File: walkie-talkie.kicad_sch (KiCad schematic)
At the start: 25 parts, among them J1 I2C, U1 ESP32-S3(R8), U10 FS-1540, U11 PJ-327A_5JJ, U12 LIS2DH12TR, U13 MCP73831T-2ACI_OT, U14 ON, U15 AP2112K-3_3TRG1, U16 +, U2 BH-18650-B1BA002, U3 mems-mic, U4 TF-115, U5 SK6812MINI-HS, U6 SK6812MINI-HS, U7 SK6812MINI-HS, U8 SK6812MINI-HS, U9 MAX98357AETE+T

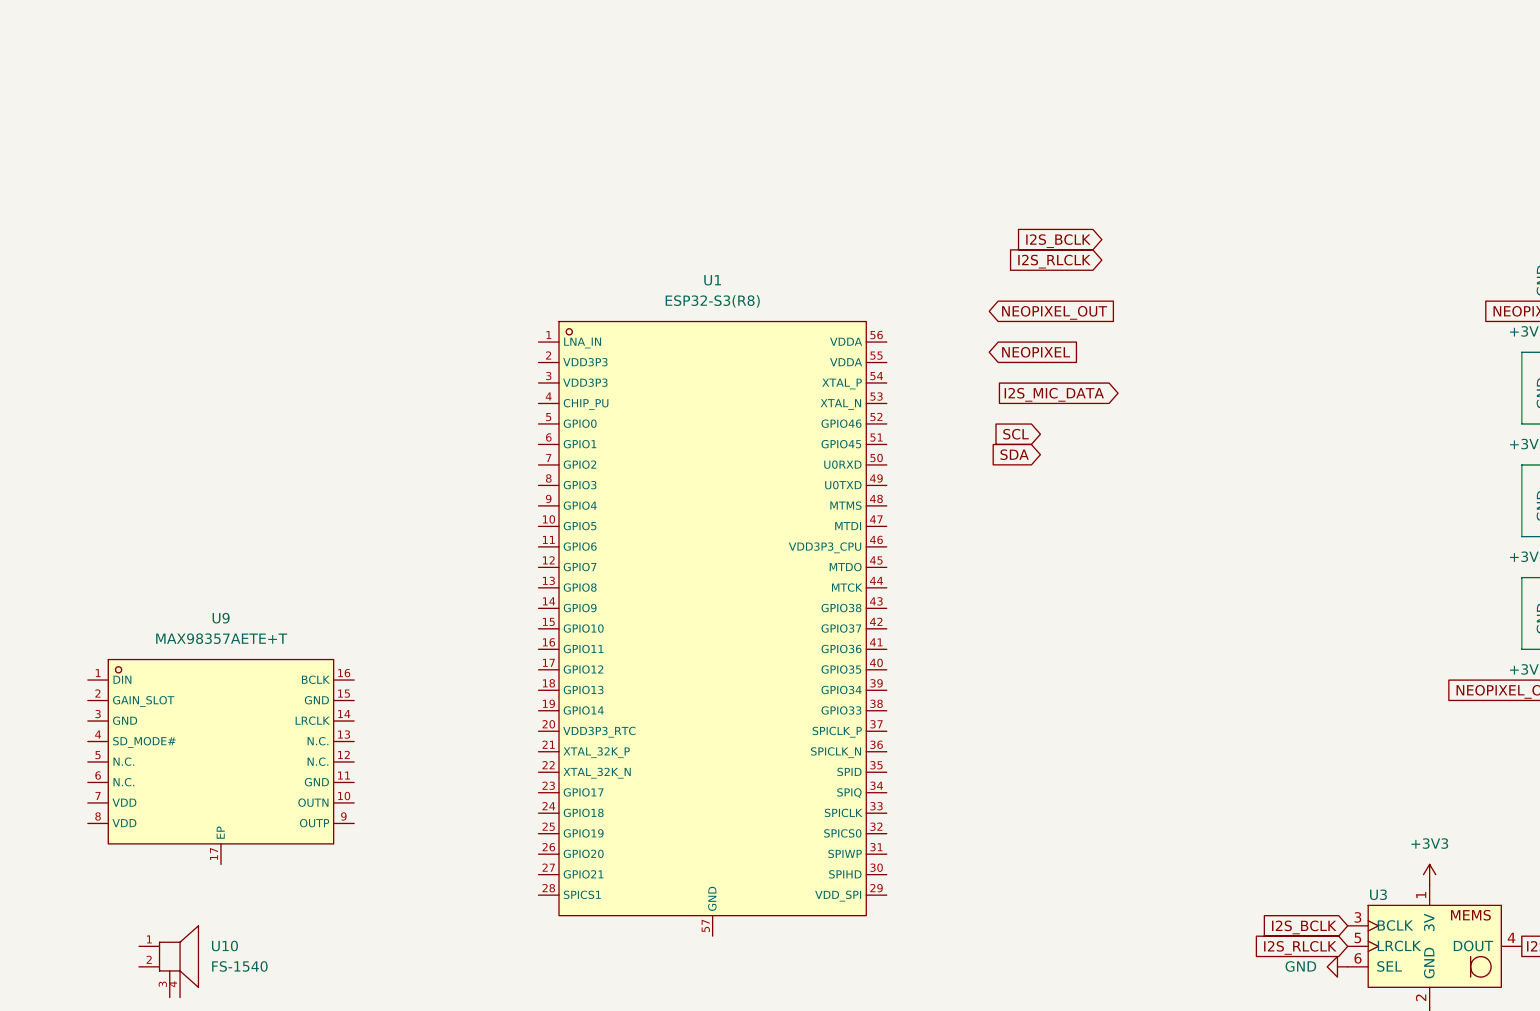
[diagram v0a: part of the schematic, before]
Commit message: WIP
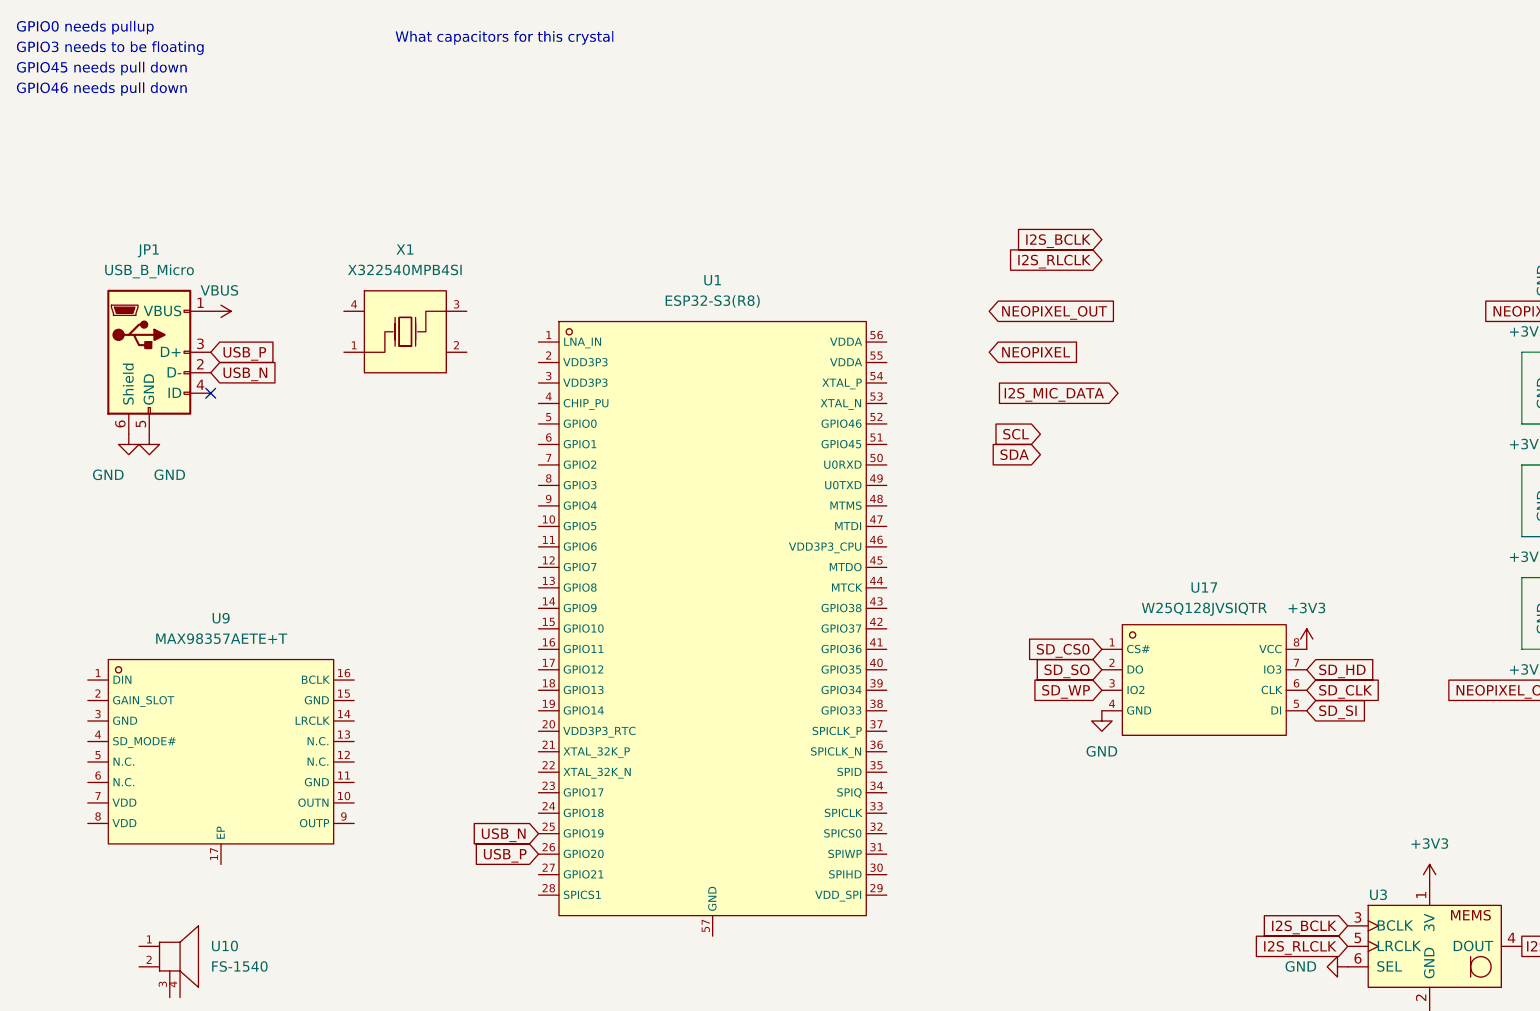
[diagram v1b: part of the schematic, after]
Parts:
- added JP1: USB_B_Micro, jlc_footprints:MICRO-USB-SMD_1050171001, symbol Connector:USB_B_Micro
- added U17: W25Q128JVSIQTR, jlc_footprints:SOIC-8_L5.3-W5.3-P1.27-LS8.0-BL, symbol jlc_symbols:W25Q128JVSIQTR
- added X1: X322540MPB4SI, jlc_footprints:OSC-SMD_4P-L3.2-W2.5-BL_SIT8008BI, symbol jlc_symbols:X322540MPB4SI
- H1, H2, H3: now left out of the parts list
- J1: footprint footprint:CONN-SMD_BM04B-SRSS-TB -> jlc_footprints:CONN-SMD_BM04B-SRSS-TB
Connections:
- net +3V3: now also U17.8 (VCC)
- net GND: now also JP1.5 (GND), JP1.6 (Shield), U17.4 (GND)
- net USB_N: now reaches U1.25 (GPIO19)
- net USB_N: now also JP1.2 (D-)
- net USB_P: now reaches U1.26 (GPIO20)
- net USB_P: now also JP1.3 (D+)
- new net SD_CLK: U17.6 (CLK)
- new net SD_CS0: U17.1 (CS#)
- new net SD_HD: U17.7 (IO3)
- new net SD_SI: U17.5 (DI)
- new net SD_SO: U17.2 (DO)
- new net SD_WP: U17.3 (IO2)
- new net VBUS: JP1.1 (VBUS)
- no-connect marks 0 -> 1
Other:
- note added: "GPIO0 needs pullup"
- note added: "GPIO3 needs to be floating"
- note added: "GPIO45 needs pull down"
- note added: "GPIO46 needs pull down"
- note added: "What capacitors for this crystal"
